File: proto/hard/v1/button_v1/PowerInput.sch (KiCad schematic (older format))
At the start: 14 parts, among them J5 USB_B_Micro, U3 AP1117-33, U4 RT8009-33, U7 RClamp0554S

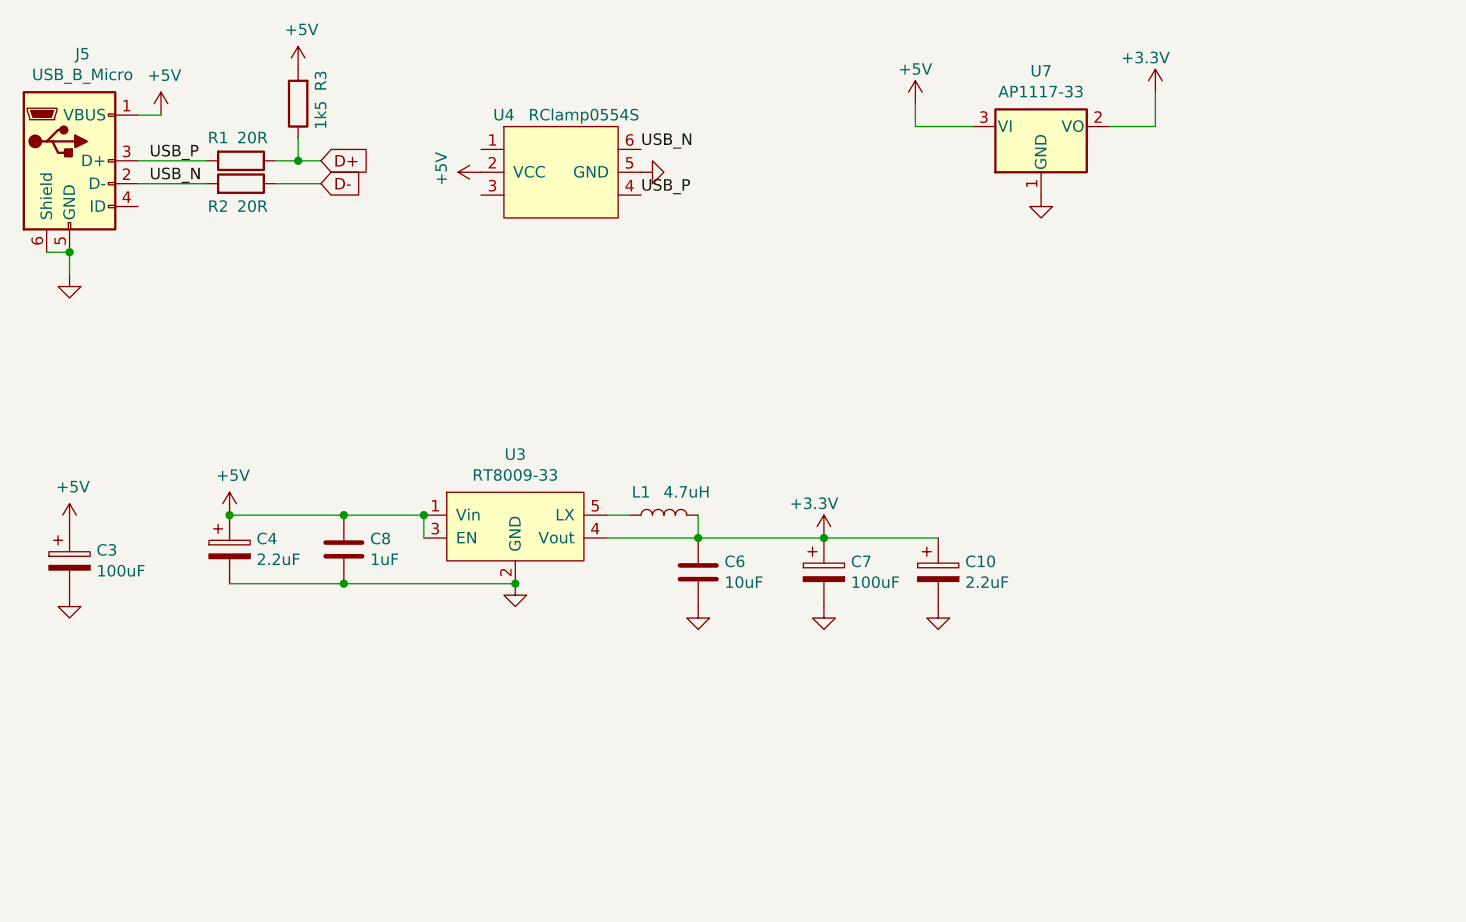
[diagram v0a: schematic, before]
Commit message: Finished main board PCB
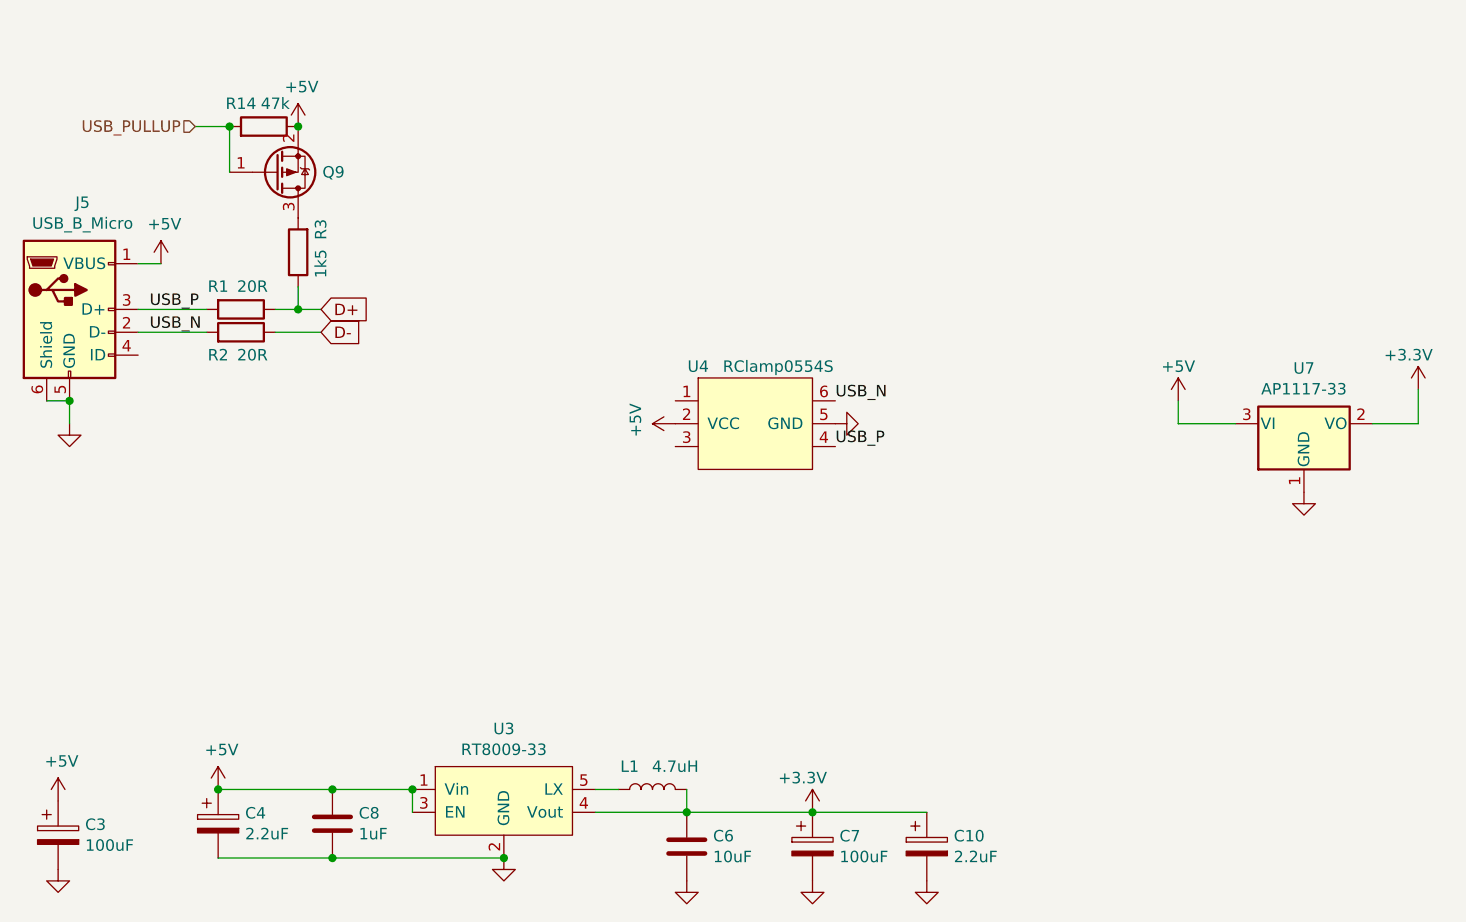
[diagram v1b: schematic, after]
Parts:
- added Q9: TP0610T, Package_TO_SOT_SMD:SOT-23, symbol Transistor_FET:TP0610T
- added R14: 47k, Resistor_SMD:R_0805_2012Metric_Pad1.15x1.40mm_HandSolder, symbol Device:R
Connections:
- net +5V: now also Q9.2 (S), R14.1; no longer R3.2
- new net: Q9.3 (D), R3.2
- new net USB_PULLUP: Q9.1 (G), R14.2
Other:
- moved on the sheet: C10, C3, C4, C6, C7, C8, J5, L1, R1, R2, R3, U3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
